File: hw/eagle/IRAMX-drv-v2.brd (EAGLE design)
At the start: 100 x 75.6 mm, 60 parts, among them IC1 IRAMTOP, IC3 LM393N, IC4 4049N, IC5 4013N, IC6 7805, IC7 7815, Q1 IRF740

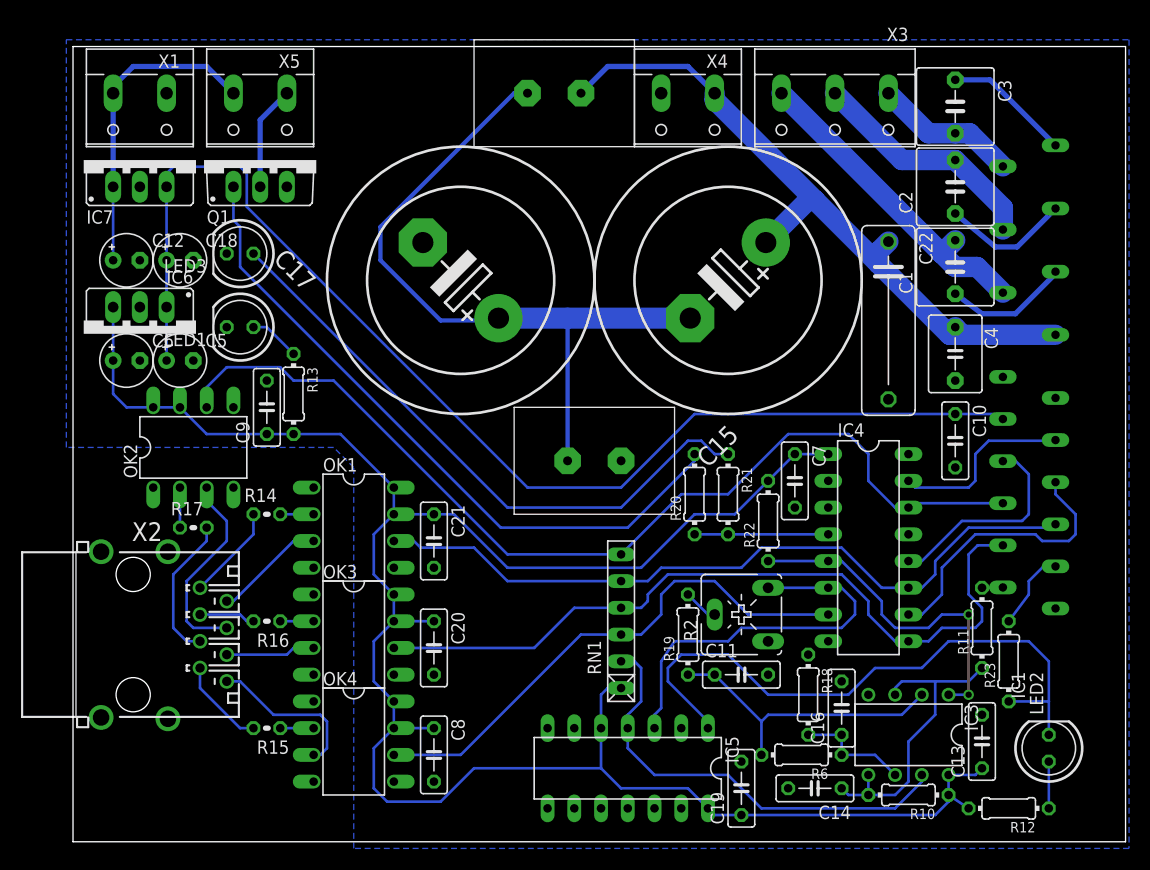
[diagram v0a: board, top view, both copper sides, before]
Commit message: hw
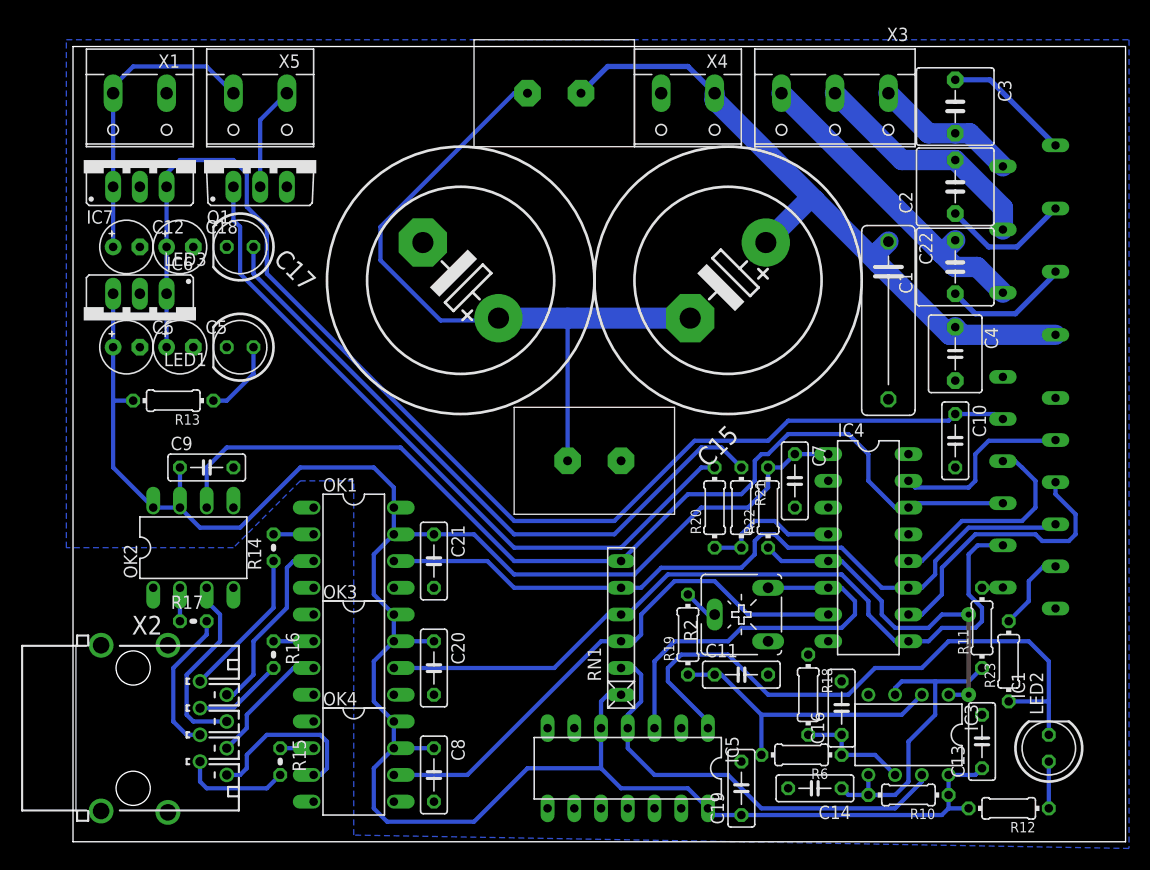
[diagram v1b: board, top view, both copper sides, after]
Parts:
- moved R13 11.4 mm to (9.53, 41.9), turned to 180 degrees
- moved OK2 9.53 mm to (11.4, 27.9)
- moved R17 8.89 mm to (11.4, 21.0)
- moved X2 8.89 mm to (5.71, 10.8)
- moved C9 8.08 mm to (12.7, 35.6), turned to 0 degrees
- moved R15 3.42 mm to (19.7, 7.62), turned to 270 degrees
- moved R14 3.24 mm to (19.1, 27.9), turned to 90 degrees
- moved R16 3.24 mm to (19.1, 17.8), turned to 270 degrees
- moved R20 2.29 mm to (61.0, 31.8)
- moved C8 1.91 mm to (34.3, 6.35)
- moved LED1 1.91 mm to (15.9, 47.0)
- moved OK4 1.91 mm to (26.7, 7.62)
- moved C20 1.90 mm to (34.3, 16.5)
- moved C21 1.90 mm to (34.3, 26.7)
- moved OK1 1.90 mm to (26.7, 27.9)
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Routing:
- net +5V: track 202.8 -> 221.5 mm
- net N$20: track 10.6 -> 17.6 mm
- net N$31: track 9.09 -> 14.3 mm
- net N$9: track 58.2 -> 63.4 mm
- net +15V: track 115.0 -> 119.5 mm
- net N$16: track 8.52 -> 12.2 mm
- net N$17: track 5.34 -> 8.56 mm
- net N$40: track 64.6 -> 67.5 mm
- net N$43: track 4.86 -> 7.40 mm
- net N$23: track 8.56 -> 10.3 mm
- net N$35: track 70.6 -> 72.1 mm
- net +24V: track 29.8 -> 28.5 mm
- net N$19: track 19.1 -> 18.0 mm
- net N$18: track 15.2 -> 16.2 mm
- net N$29: track 50.5 -> 51.3 mm
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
